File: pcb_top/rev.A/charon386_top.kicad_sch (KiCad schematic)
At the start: 151 parts, among them J1 PJ-322, J2 Vol. Btns, J3 Conn_02x07_Odd_Even, J4 ESP, J5 PC104_16, J6 PC104, SW1 VGA Config, U1 74HC4050, U10 AMS1117-5.0, U11 MT4C4256, U12 MT4C4256, U13 MT4C4256, U14 MT4C4256, U2 NE5532DR, U3 74HCT138, U4 ES1868F, U5 TVGA9000I, U6 SAM2695, U7 27C256, U8 AMS1117-5.0, U9 AMS1117-3.3, Y1 40 MHz, Y2 12 MHz

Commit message: wip pcb rev.A
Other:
- company: (none) -> Eugene Lozovoy
- title: (none) -> PC-CHARON-386-TOP
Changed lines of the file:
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@@
   (paper "User" 599.999 350.012)
   (title_block
+    (title "PC-CHARON-386-TOP")
     (date "2021-12-17")
     (rev "A")
+    (company "Eugene Lozovoy")
+    (comment 1 "VGA & Sound board for Charon-386")
   )
   (junction (at 465.455 292.735) (diameter 1.016) (color 0 0 0 0)

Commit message: wip pcb rev.A (almost done now)
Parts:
- SW1: footprint Button_Switch_THT:SW_DIP_SPSTx02_Slide_9.78x7.26mm_W7.62mm_P2.54mm -> Button_Switch_THT:SW_DIP_SPSTx02_Slide_6.7x6.64mm_W7.62mm_P2.54mm_LowProfile
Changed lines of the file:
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@@
       (effects (font (size 1 1)))
     )
-    (property "Footprint" "Button_Switch_THT:SW_DIP_SPSTx02_Slide_9.78x7.26mm_W7.62mm_P2.54mm" (id 2) (at 214.63 147.955 0)
+    (property "Footprint" "Button_Switch_THT:SW_DIP_SPSTx02_Slide_6.7x6.64mm_W7.62mm_P2.54mm_LowProfile" (id 2) (at 214.63 147.955 0)
       (effects (font (size 1.27 1.27)) hide)
     )
@@
     )
     (path "/46d8c6f2-9c28-4bc8-bf83-68eb4225e4b8"
-      (reference "SW1") (unit 1) (value "VGA Config") (footprint "Button_Switch_THT:SW_DIP_SPSTx02_Slide_9.78x7.26mm_W7.62mm_P2.54mm")
+      (reference "SW1") (unit 1) (value "VGA Config") (footprint "Button_Switch_THT:SW_DIP_SPSTx02_Slide_6.7x6.64mm_W7.62mm_P2.54mm_LowProfile")
     )
     (path "/e9bb9582-e2bc-46cd-b4a2-96539521344a"

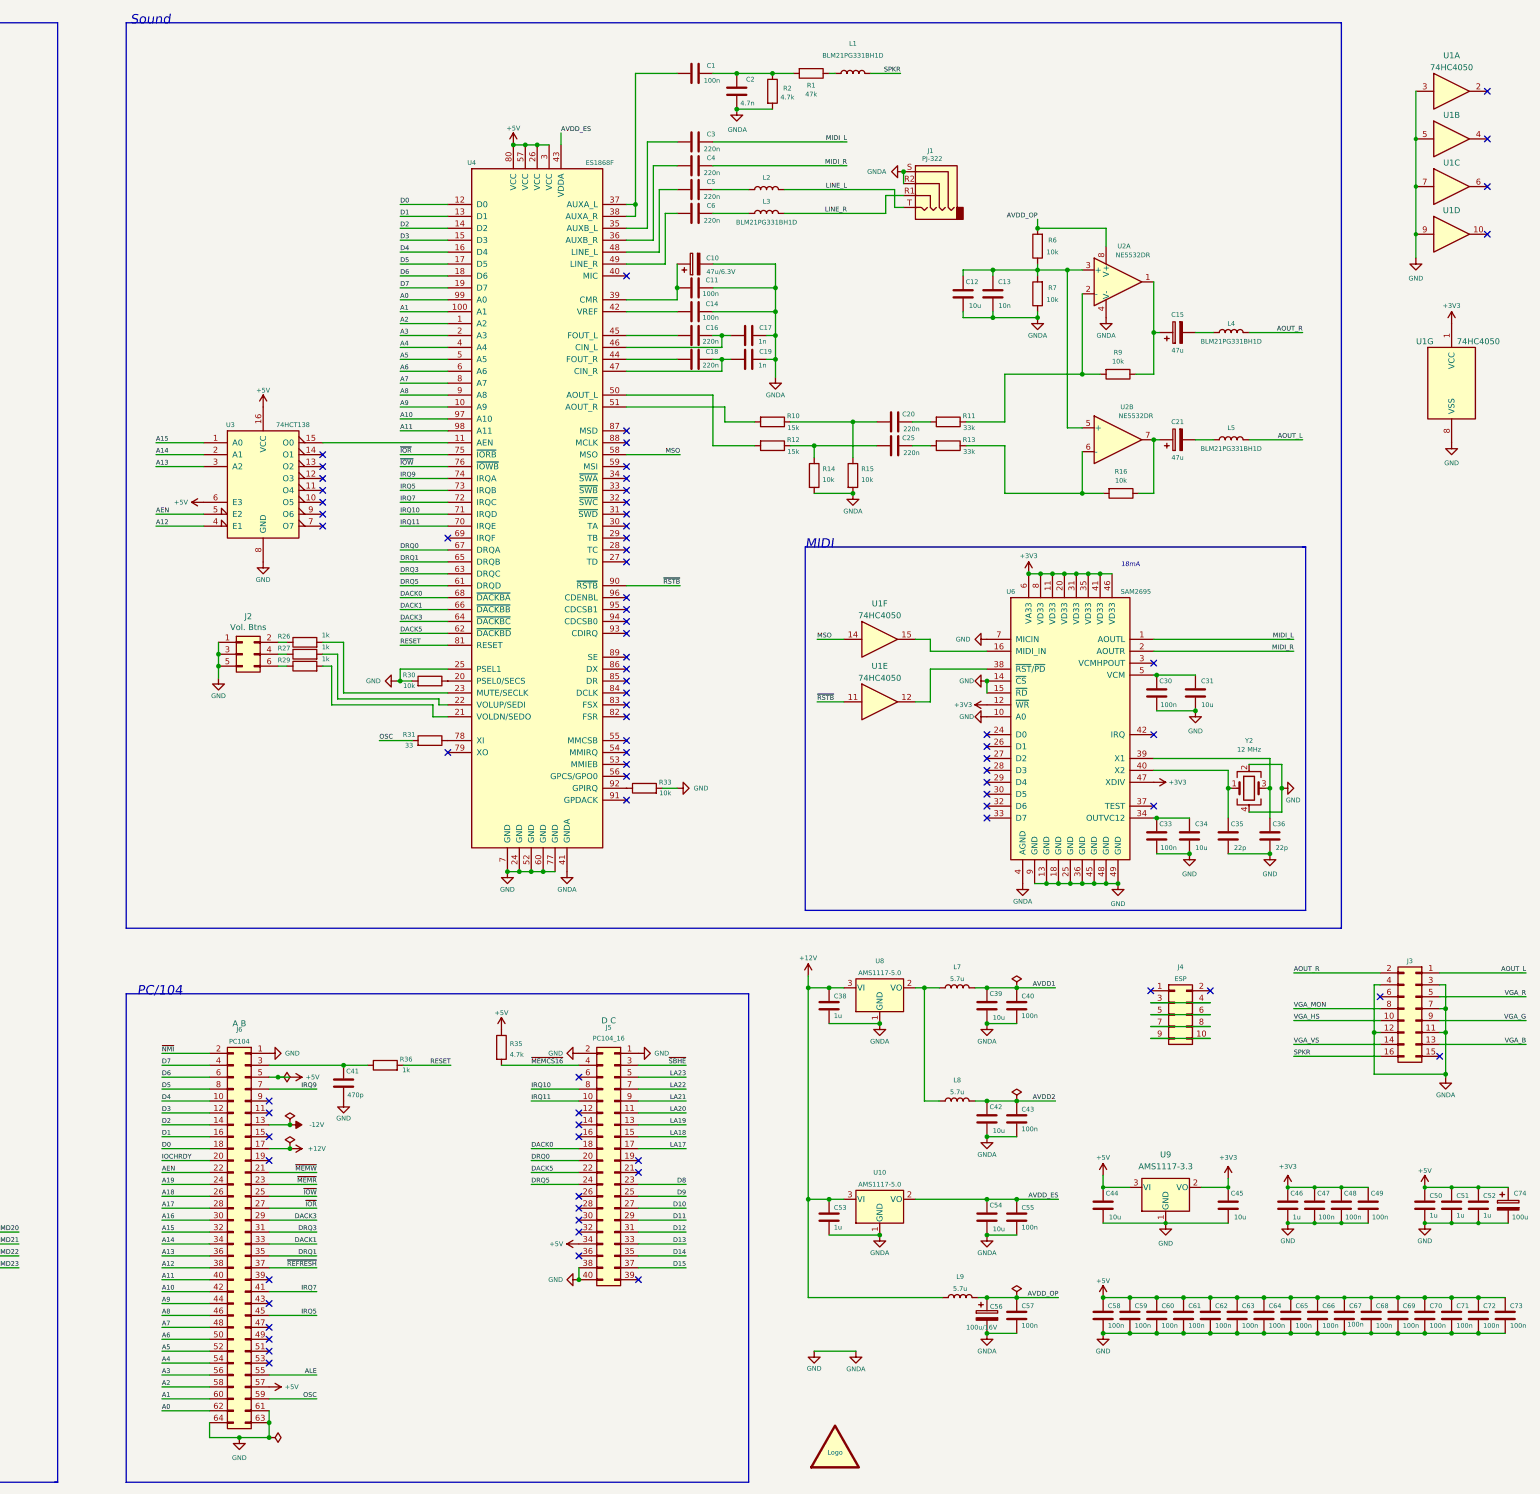
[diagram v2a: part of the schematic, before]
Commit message: wip pcb rev.A
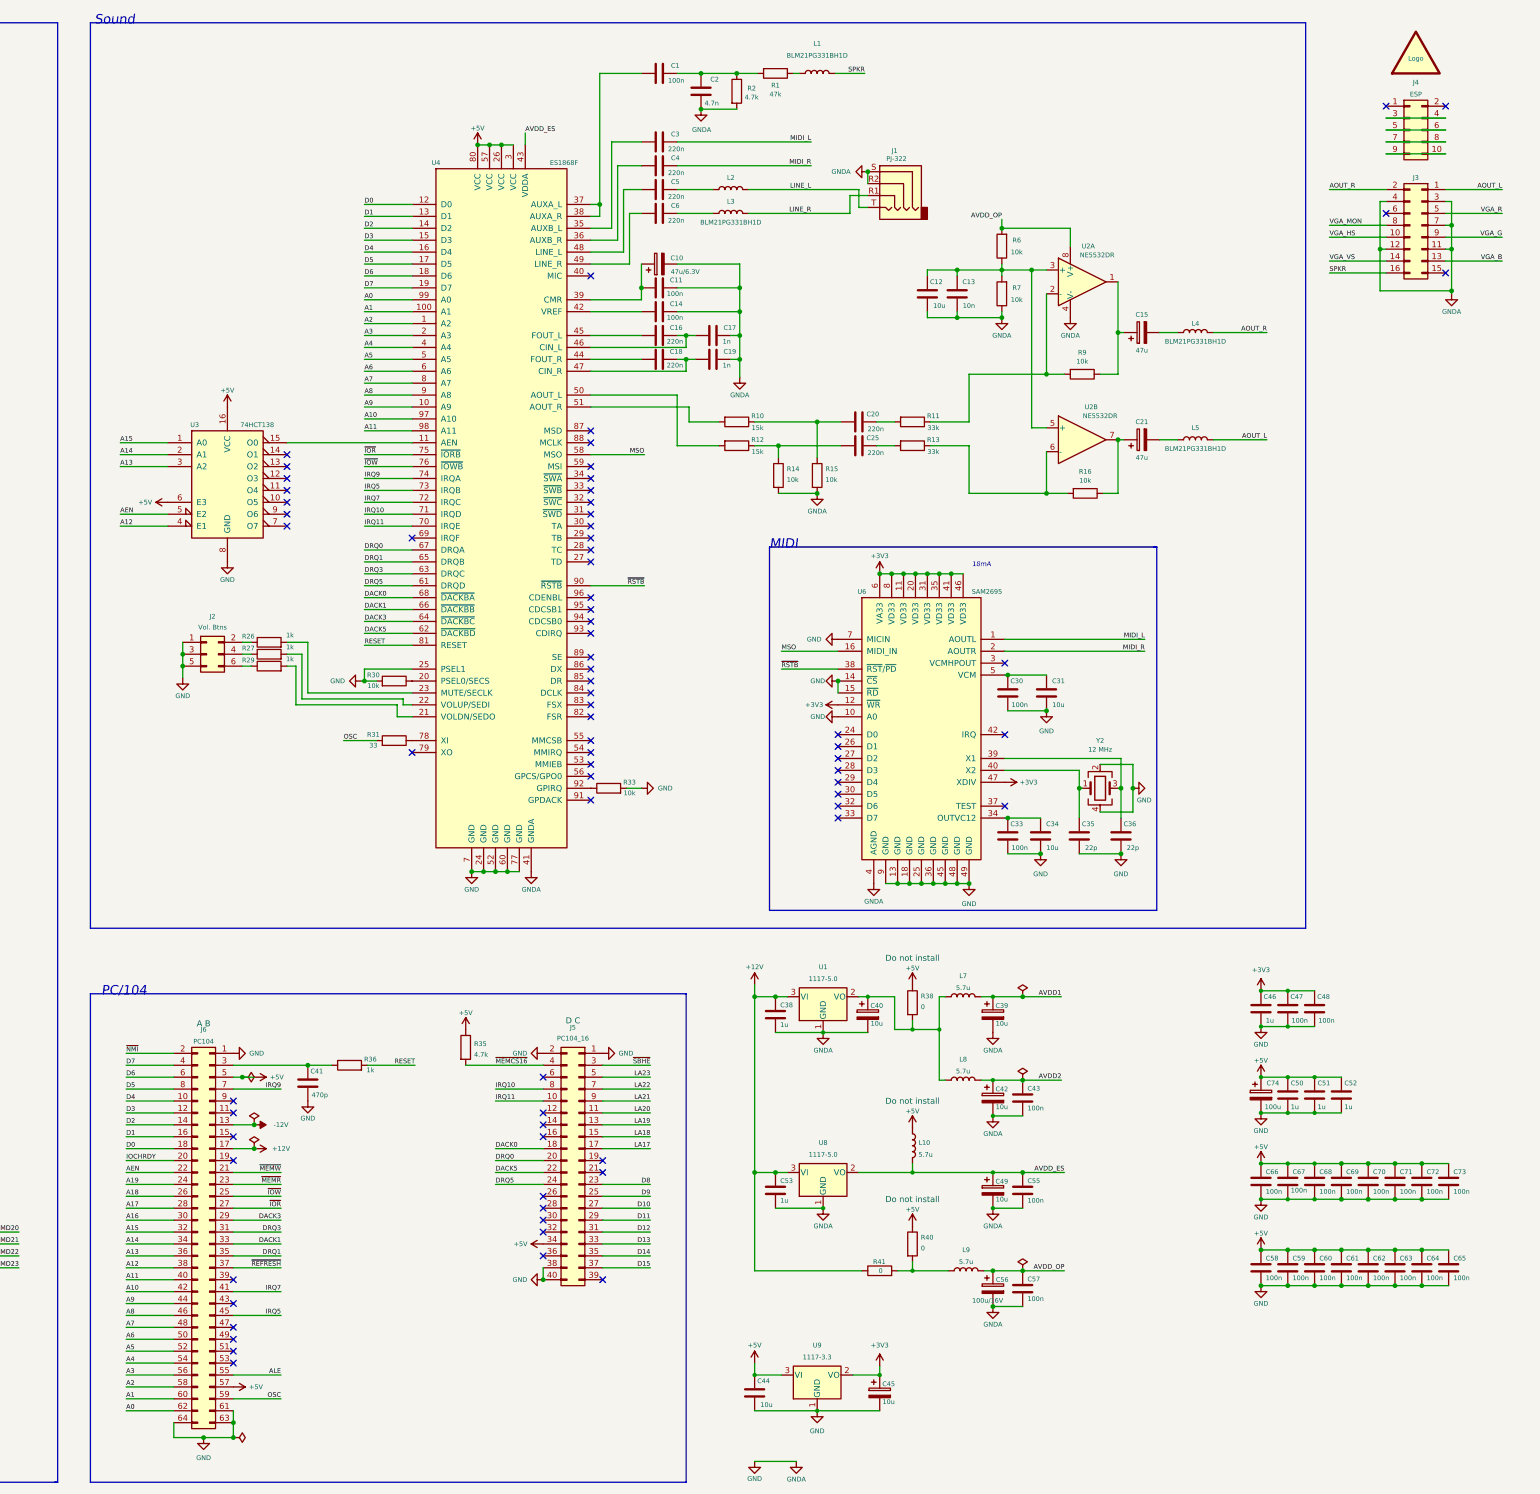
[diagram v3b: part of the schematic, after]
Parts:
- removed C39, C42, C45, C54: 10u, Capacitor_SMD:C_0805_2012Metric_Pad1.18x1.45mm_HandSolder, symbol Device:C
- removed C40, C49: 100n, Capacitor_SMD:C_0603_1608Metric_Pad1.08x0.95mm_HandSolder, symbol Device:C
- removed U1: 74HC4050, Package_SO:SO-16_3.9x9.9mm_P1.27mm, symbol 4xxx:4050
- removed U10: AMS1117-5.0, Package_TO_SOT_SMD:SOT-223-3_TabPin2, symbol Regulator_Linear:AMS1117-5.0
- added C39, C40, C42, C45, C49: 10u, Capacitor_Tantalum_SMD:CP_EIA-3216-18_Kemet-A_Pad1.58x1.35mm_HandSolder, symbol Device:CP
- added L10: 5.7u, Inductor_SMD:L_1210_3225Metric_Pad1.42x2.65mm_HandSolder, symbol Device:L
- added R38, R40, R41: 0, Resistor_SMD:R_0805_2012Metric_Pad1.20x1.40mm_HandSolder, symbol Device:R
- added U1: 1117-5.0, Package_TO_SOT_SMD:SOT-223-3_TabPin2, symbol Regulator_Linear:AMS1117-5.0
- U8: value AMS1117-5.0 -> 1117-5.0
- U9: value AMS1117-3.3 -> 1117-3.3
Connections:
- net +12V: now also R41.1, U1.3 (VI); no longer L9.1
- net +3V3: now also C45.1
- net +5V: now also L10.1, R38.1, R40.1
- net AVDD1: now also C39.1
- net AVDD2: now also C42.1
- net AVDD_ES: now also U8.2 (VO), C49.1, L10.2
- net GND: now also C39.2, C40.2, C42.2, C45.2, C49.2, U1.1 (GND)
- net MSO: now also U6.16 (MIDI_IN)
- net ~{RSTB}: now also U6.38 (~{RST}/~{PD})
- net at L7.1, L8.1: now also C40.1, R38.2, U1.2 (VO); no longer U8.2 (VO)
- new net: L9.1, R40.2, R41.2
- no-connect marks 92 -> 88
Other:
- moved on the sheet: C1, C10, C11, C12, C13, C14, C15, C16, C17, C18, C19, C2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
